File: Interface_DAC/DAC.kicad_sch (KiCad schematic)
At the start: 14 parts, among them U5 PCM1794A

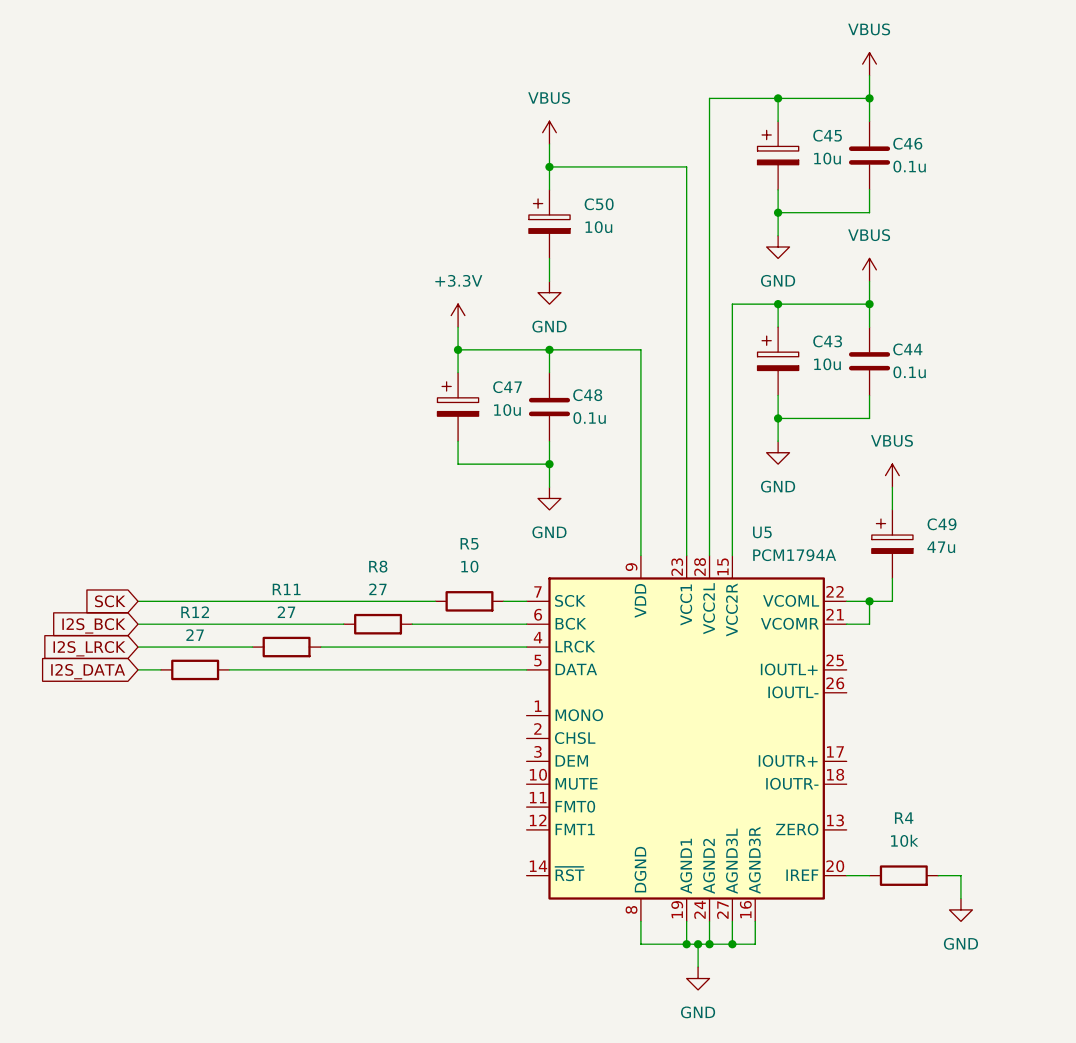
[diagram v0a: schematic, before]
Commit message: Schematic Tinkering and PCB Layout
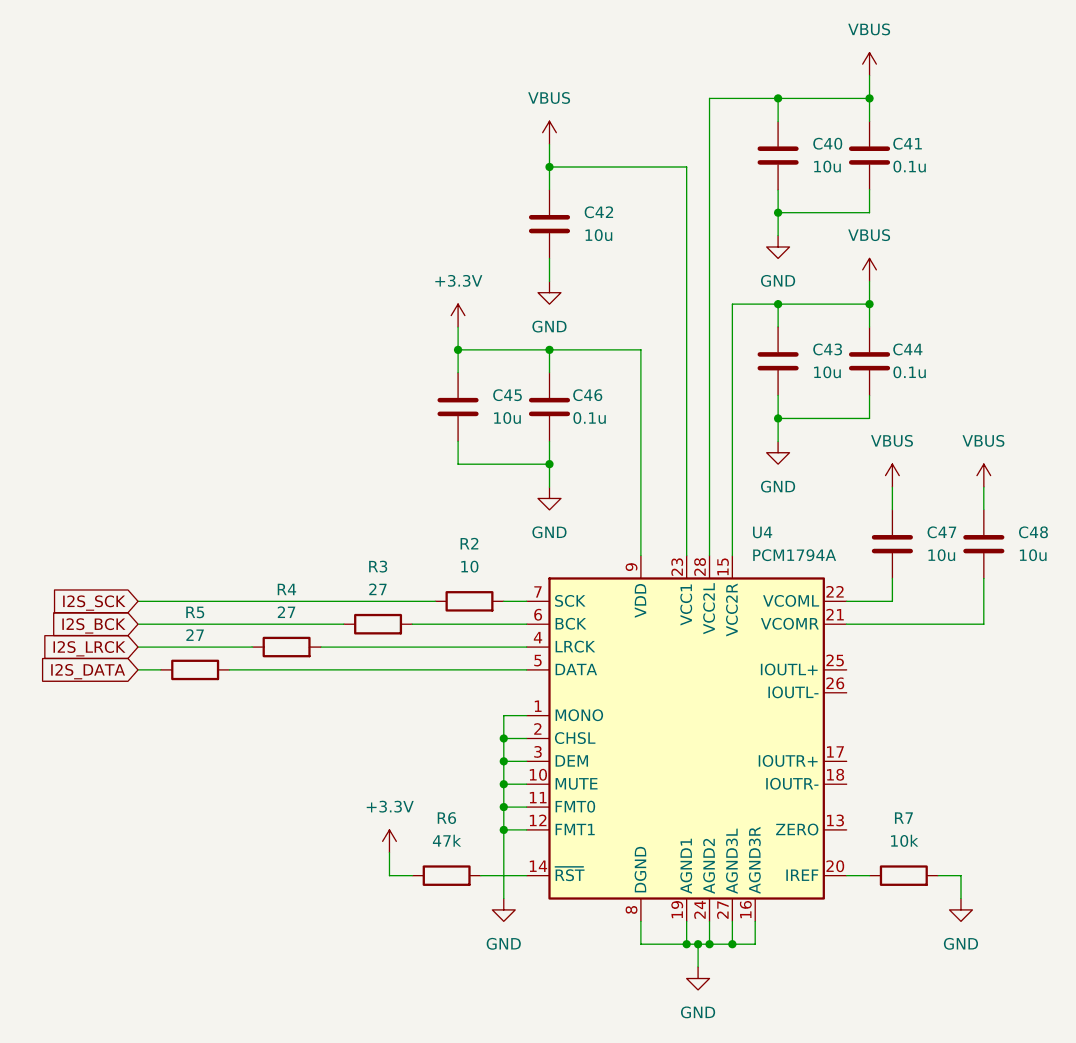
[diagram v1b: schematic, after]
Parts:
- added C48: 10u, Capacitor_SMD:C_0402_1005Metric, symbol Device:C
- added R6: 47k, Resistor_SMD:R_0402_1005Metric, symbol Device:R
- C40: renamed from C45; footprint Capacitor_Tantalum_SMD:CP_EIA-2012-12_Kemet-R -> Capacitor_SMD:C_0402_1005Metric; symbol Device:C_Polarized -> Device:C
- C42: renamed from C50; footprint Capacitor_Tantalum_SMD:CP_EIA-2012-12_Kemet-R -> Capacitor_SMD:C_0402_1005Metric; symbol Device:C_Polarized -> Device:C
- C43: footprint Capacitor_Tantalum_SMD:CP_EIA-2012-12_Kemet-R -> Capacitor_SMD:C_0402_1005Metric; symbol Device:C_Polarized -> Device:C
- C45: renamed from C47; footprint Capacitor_Tantalum_SMD:CP_EIA-2012-12_Kemet-R -> Capacitor_SMD:C_0402_1005Metric; symbol Device:C_Polarized -> Device:C
- C47: renamed from C49; value 47u -> 10u; footprint Capacitor_Tantalum_SMD:CP_EIA-3216-18_Kemet-A -> Capacitor_SMD:C_0402_1005Metric; symbol Device:C_Polarized -> Device:C
- renumbered C46 to C41, C48 to C46, R5 to R2, R8 to R3, R11 to R4, R12 to R5, R4 to R7, U5 to U4
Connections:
- net +3.3V: now also R6.1
- net GND: now also U4.1 (MONO), U4.10 (MUTE), U4.11 (FMT0), U4.12 (FMT1), U4.2 (CHSL), U4.3 (DEM)
- net VBUS: now also C48.1
- net at C47.2, U4.22 (VCOML): no longer U4.21 (VCOMR)
- net at U4.14 (~{RST}): now also R6.2
- net SCK renamed I2S_SCK
- new net: C48.2, U4.21 (VCOMR)
